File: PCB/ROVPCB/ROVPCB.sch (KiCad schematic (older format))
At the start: 15 parts, among them J1 Conn_01x04_Male, J2 Conn_01x04_Male, P1 Conn_02x20_Odd_Even, U1 MPU-9250, U2 BME280, U3 LIGHT_TSL2591, U4 LTC4316IDDPBF

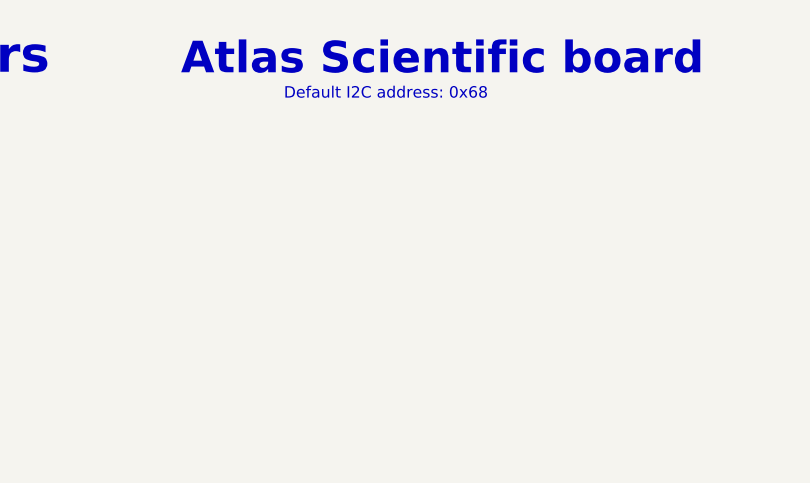
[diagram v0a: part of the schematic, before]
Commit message: Adding the Atlas Board... BNC??
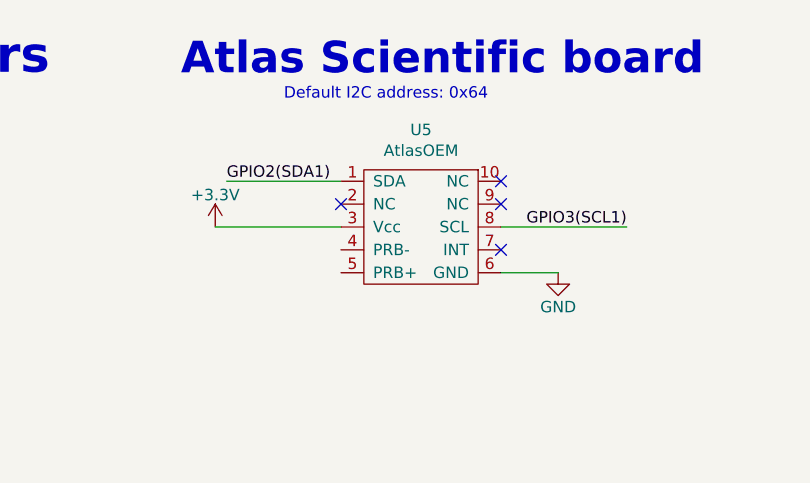
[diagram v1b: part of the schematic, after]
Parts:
- added U5: AtlasOEM, Adafruit TSL2591:OEM Board, symbol Adafruit_TSL2591-eagle-import:AtlasOEM
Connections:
- net +3V3: now also U5.3 (Vcc)
- net GND: now also U5.6 (GND)
- net GPIO2(SDA1): now also U5.1 (SDA)
- net GPIO3(SCL1): now also U5.8 (SCL)
- no-connect marks 31 -> 35
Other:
- note added: "Default I2C address: 0x64"
- note removed: "Default I2C address: 0x68"
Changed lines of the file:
@@
 	7000 5250 7500 5250
 $Comp
-L ROVPCB-rescue:GND-power-ROVPCB-rescue-ROVPCB-rescue #PWR?
+L ROVPCB-rescue:GND-power-ROVPCB-rescue-ROVPCB-rescue #PWR0111
 U 1 1 5CB8FA80
 P 7500 6000
-F 0 "#PWR?" H 7500 5750 50  0001 C CNN
+F 0 "#PWR0111" H 7500 5750 50  0001 C CNN
 F 1 "GND" H 7500 5850 50  0000 C CNN
 F 2 "" H 7500 6000 50  0000 C CNN
@@
 	6750 5450 7500 5450
 $Comp
-L ROVPCB-rescue:GND-power-ROVPCB-rescue-ROVPCB-rescue #PWR?
+L ROVPCB-rescue:GND-power-ROVPCB-rescue-ROVPCB-rescue #PWR0112
 U 1 1 5CBA3506
 P 9250 5550
-F 0 "#PWR?" H 9250 5300 50  0001 C CNN
+F 0 "#PWR0112" H 9250 5300 50  0001 C CNN
 F 1 "GND" H 9250 5400 50  0000 C CNN
 F 2 "" H 9250 5550 50  0000 C CNN
@@
 	9250 5550 9150 5550
 $Comp
-L ROVPCB-rescue:+3.3V-power-ROVPCB-rescue-ROVPCB-rescue #PWR?
+L ROVPCB-rescue:+3.3V-power-ROVPCB-rescue-ROVPCB-rescue #PWR0113
 U 1 1 5CBA6BEC
 P 9350 5350
-F 0 "#PWR?" H 9350 5200 50  0001 C CNN
+F 0 "#PWR0113" H 9350 5200 50  0001 C CNN
 F 1 "+3.3V" H 9350 5490 50  0000 C CNN
 F 2 "" H 9350 5350 50  0000 C CNN
@@
 Default I2C address: 0x29
 Text Notes 8050 900  0    50   ~ 0
-Default I2C address: 0x68
+Default I2C address: 0x64
 Text Notes 4550 900  0    50   ~ 0
 Default I2C address--Temp: 0x77; Pressure: 0x76
 $Comp
-L ROVPCB-rescue:GND-power-ROVPCB-rescue-ROVPCB-rescue #PWR?
+L ROVPCB-rescue:GND-power-ROVPCB-rescue-ROVPCB-rescue #PWR0114
 U 1 1 5CBDF2B2
 P 6200 4900
-F 0 "#PWR?" H 6200 4650 50  0001 C CNN
+F 0 "#PWR0114" H 6200 4650 50  0001 C CNN
 F 1 "GND" H 6200 4750 50  0000 C CNN
 F 2 "" H 6200 4900 50  0000 C CNN
@@
 	1    0    0    -1
 $EndComp
+$Comp
+L Adafruit_TSL2591-eagle-import:AtlasOEM U5
+U 1 1 5CBE687D
+P 8650 1400
+F 0 "U5" H 8650 1775 50  0000 C CNN
+F 1 "AtlasOEM" H 8650 1684 50  0000 C CNN
+F 2 "Adafruit TSL2591:OEM Board" H 8650 1400 50  0001 C CNN
+F 3 "https://www.atlas-scientific.com/_files/_datasheets/_oem/EC_oem_datasheet.pdf" H 8650 1400 50  0001 C CNN
+	1    8650 1400
+	1    0    0    -1
+$EndComp
+NoConn ~ 9000 1250
+NoConn ~ 9000 1350
+NoConn ~ 8300 1350
+Text Label 7800 1250 0    50   ~ 0
+GPIO2(SDA1)
+Wire Wire Line
+	7800 1250 8300 1250
+Text Label 9550 1450 2    50   ~ 0
+GPIO3(SCL1)
+Wire Wire Line
+	9550 1450 9000 1450
+$Comp
+L ROVPCB-rescue:GND-power-ROVPCB-rescue-ROVPCB-rescue #PWR?
+U 1 1 5CBFDF85
+P 9250 1650
+F 0 "#PWR?" H 9250 1400 50  0001 C CNN
+F 1 "GND" H 9250 1500 50  0000 C CNN
+F 2 "" H 9250 1650 50  0000 C CNN
+F 3 "" H 9250 1650 50  0000 C CNN
+	1    9250 1650
+	1    0    0    -1
+$EndComp
+Wire Wire Line
+	9250 1650 9000 1650
+$Comp
+L ROVPCB-rescue:+3.3V-power-ROVPCB-rescue-ROVPCB-rescue #PWR?
+U 1 1 5CC01F57
+P 7750 1450
+F 0 "#PWR?" H 7750 1300 50  0001 C CNN
+F 1 "+3.3V" H 7750 1590 50  0000 C CNN
+F 2 "" H 7750 1450 50  0000 C CNN
+F 3 "" H 7750 1450 50  0000 C CNN
+	1    7750 1450
+	1    0    0    -1
+$EndComp
+Wire Wire Line
+	7750 1450 8300 1450
+NoConn ~ 9000 1550
 $EndSCHEMATC
